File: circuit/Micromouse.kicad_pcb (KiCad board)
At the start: 2 copper layers, 78 x 100 mm, 84 parts, among them CN1 Battery, CN2 Battery, J1 DBG_CN, J3 TEST_1P, J5 TEST_1P, J6 Conn_01x04, J7 Conn_02x03_Odd_Even, J8 Conn_02x03_Odd_Even, Q1 IRLML6402, Q2 IRLML6344, Q3 ST-1KL3A, Q5 ST-1KL3A, Q7 ST-1KL3A, Q9 ST-1KL3A, SW1 SW_SPDT, SW2 SW_Push, SW3 SW_Push, SW4 SW_Push, U1 NJM7805S, U2 TB6612FNG, U3 STM32F405RGTx, U4 ADP7182AUJZ-3.3, U5 AD8397, U6 AD8397, U7 ICM-20602-module

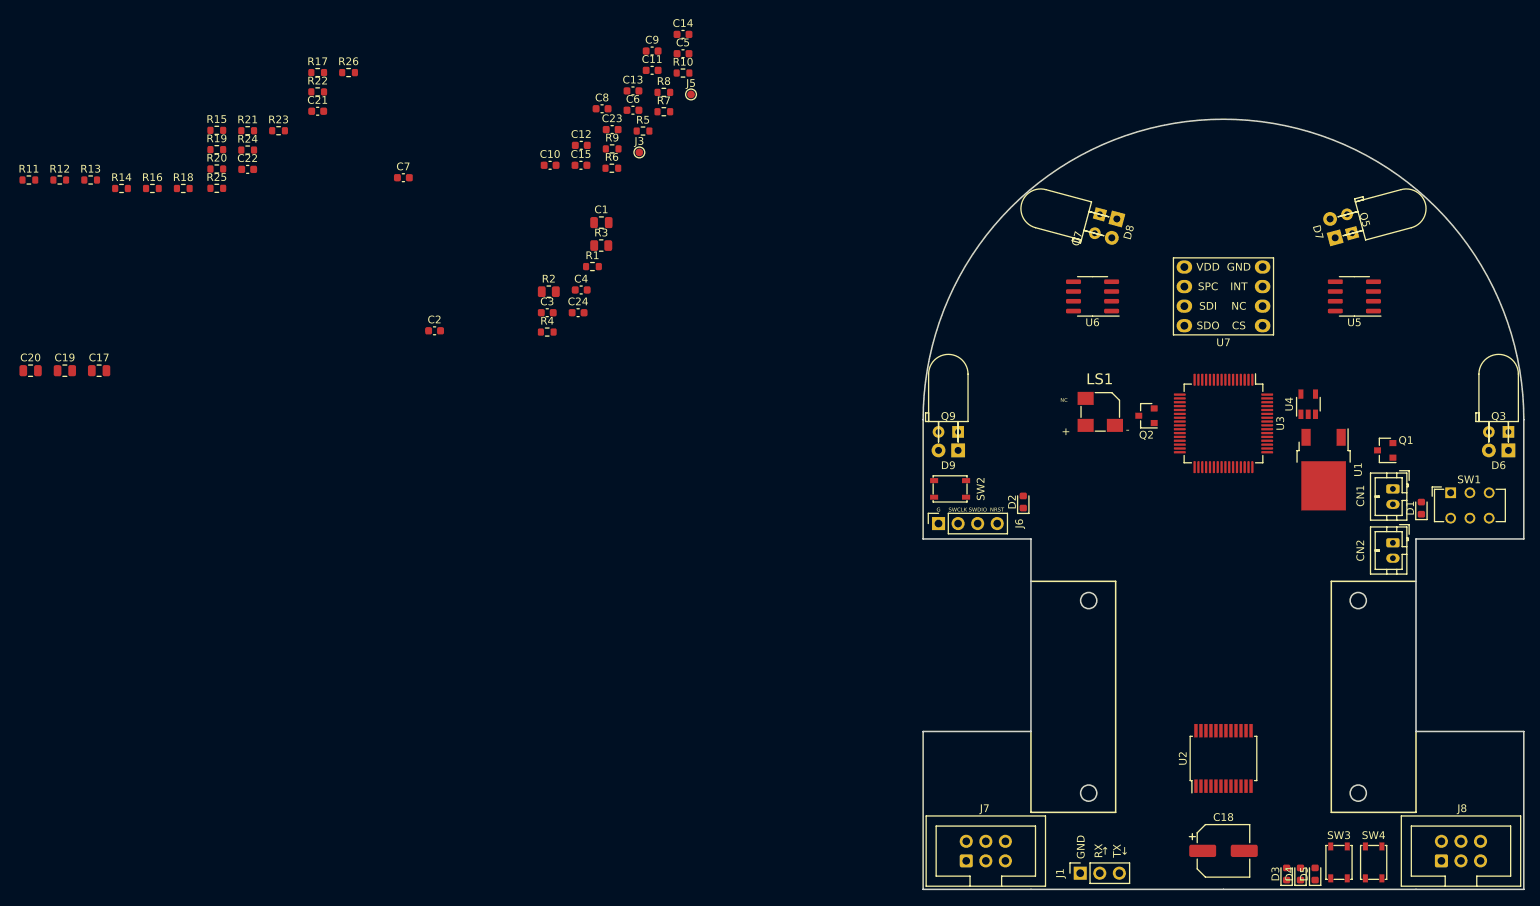
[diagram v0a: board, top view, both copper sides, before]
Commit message: 何となーくの部品配置
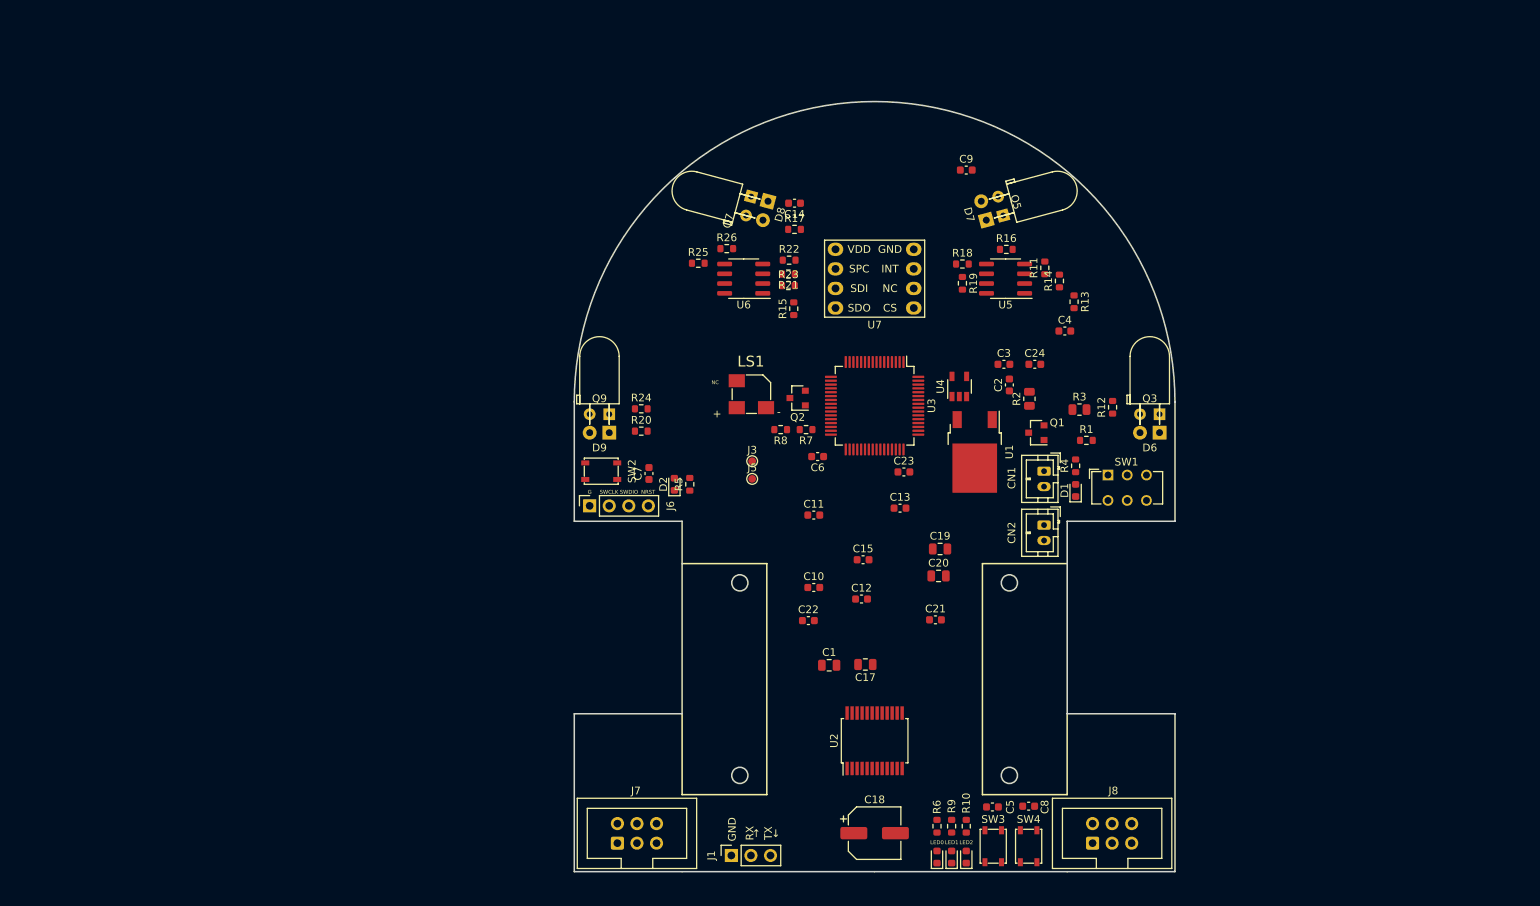
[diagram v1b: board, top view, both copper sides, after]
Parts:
- moved R12 139.9 mm to (175.6, 82.4), turned to 90 degrees
- moved R11 132.4 mm to (166.8, 64.3), turned to 90 degrees
- moved R13 128.7 mm to (170.6, 68.7), turned to 270 degrees
- moved R14 122.4 mm to (168.7, 66.0), turned to 90 degrees
- moved C20 120.9 mm to (153.0, 104.3)
- moved C19 116.0 mm to (153.2, 100.8)
- moved R16 111.2 mm to (161.8, 61.9)
- moved C17 106.6 mm to (143.5, 115.8), turned to 180 degrees
- moved C8 106.2 mm to (164.7, 134.2), turned to 180 degrees
- moved C5 105.7 mm to (160.0, 134.3), turned to 180 degrees
- moved R10 104.5 mm to (156.6, 136.8), turned to 270 degrees
- moved C21 103.9 mm to (152.6, 110.0)
- moved R18 101.6 mm to (156.1, 63.8)
- moved R9 98.4 mm to (154.7, 136.8), turned to 270 degrees
- moved R19 98.4 mm to (156.1, 66.3), turned to 270 degrees
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- renumbered D3 to LED0, D4 to LED1, D5 to LED2
